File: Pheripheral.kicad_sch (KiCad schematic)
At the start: 19 parts

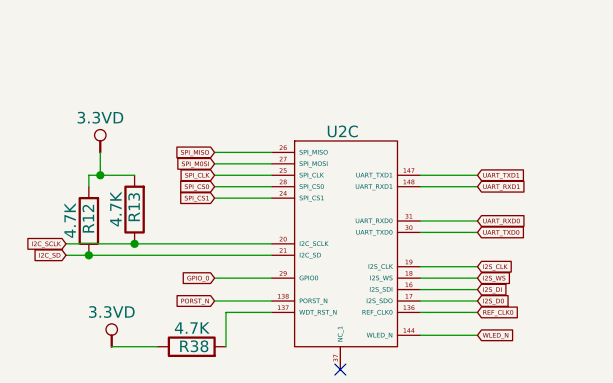
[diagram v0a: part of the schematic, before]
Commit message: f_ver
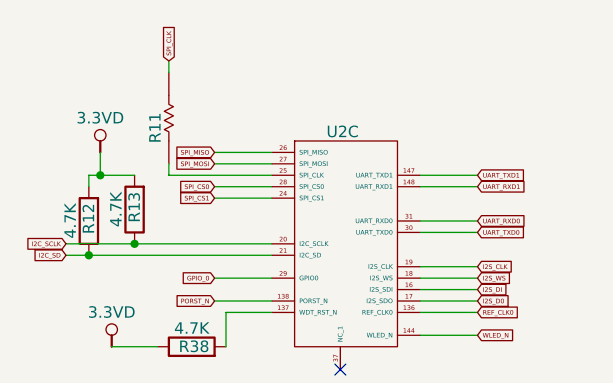
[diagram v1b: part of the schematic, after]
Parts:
- added R11: 22, Resistor_SMD:R_0402_1005Metric, symbol MT7688AN_Reset-altium-import:root_2_Res1_Miscellaneous Devices.SchLib
- U2: footprint MT7628:MT7628_footprint -> Library:MT7628_footprint
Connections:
- net SPI_CLK: now also R11.1; no longer U2.25 (SPI_CLK)
- net SPI_M0SI renamed SPI_MOSI
- new net: R11.2, U2.25 (SPI_CLK)
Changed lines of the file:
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@@
 	(wire
 		(pts
+			(xy 43.18 29.21) (xy 43.18 30.48)
+		)
+		(stroke
+			(width 0)
+			(type default)
+		)
+	)
+	(wire
+		(pts
 			(xy 31.75 39.37) (xy 34.29 39.37)
 		)
@@
 	(wire
 		(pts
+			(xy 43.18 17.78) (xy 43.18 19.05)
+		)
+		(stroke
+			(width 0)
+			(type default)
+		)
+	)
+	(wire
+		(pts
 			(xy 115.57 34.29) (xy 127 34.29)
 		)
@@
 	(wire
 		(pts
+			(xy 43.18 30.48) (xy 54.61 30.48)
+		)
+		(stroke
+			(width 0)
+			(type default)
+		)
+	)
+	(wire
+		(pts
 			(xy 149.86 29.21) (xy 152.4 29.21)
 		)
@@
 	(wire
 		(pts
-			(xy 48.26 30.48) (xy 54.61 30.48)
-		)
-		(stroke
-			(width 0)
-			(type default)
-		)
-	)
-	(wire
-		(pts
 			(xy 48.26 33.02) (xy 54.61 33.02)
 		)
@@
 		)
 	)
-	(global_label "SPI_M0SI"
+	(global_label "SPI_MOSI"
 		(shape input)
 		(at 48.26 29.21 180)
@@
 		)
 		(property "Intersheetrefs" "${INTERSHEET_REFS}"
-			(at 43.6551 29.21 0)
+			(at 43.6067 29.21 0)
 			(effects
 				(font
@@
 	(global_label "SPI_CLK"
 		(shape input)
-		(at 48.26 30.48 180)
+		(at 43.18 17.78 90)
 		(fields_autoplaced yes)
 		(effects
@@
 				(size 0.508 0.508)
 			)
-			(justify right)
+			(justify left)
 		)
 		(property "Intersheetrefs" "${INTERSHEET_REFS}"
-			(at 44.018 30.48 0)
+			(at 43.18 13.538 90)
 			(effects
 				(font
 					(size 1.27 1.27)
 				)
-				(justify right)
+				(justify left)
 				(hide yes)
 			)
@@
 			)
 		)
-		(property "Footprint" "MT7628:MT7628_footprint"
+		(property "Footprint" "Library:MT7628_footprint"
 			(at 62.23 27.94 0)
 			(effects
@@
 			)
 		)
-		(property "Footprint" "MT7628:MT7628_footprint"
+		(property "Footprint" "Library:MT7628_footprint"
 			(at 163.83 43.18 0)
 			(effects
@@
 	)
 	(symbol
+		(lib_id "MT7688AN_Reset-altium-import:root_2_Res1_Miscellaneous Devices.SchLib")
+		(at 45.72 21.59 90)
+		(unit 1)
+		(exclude_from_sim no)
+		(in_bom yes)
+		(on_board yes)
+		(dnp no)
+		(property "Reference" "R11"
+			(at 42.418 26.924 0)
+			(effects
+				(font
+					(size 1.27 1.27)
+				)
+				(justify left bottom)
+			)
+		)
+		(property "Value" "22"
+			(at 42.418 29.718 0)
+			(effects
+				(font
+					(size 1.27 1.27)
+				)
+				(justify left bottom)
+				(hide yes)
+			)
+		)
+		(property "Footprint" "Resistor_SMD:R_0402_1005Metric"
+			(at 45.72 21.59 0)
+			(effects
+				(font
+					(size 1.27 1.27)
+				)
+				(hide yes)
+			)
+		)
+		(property "Datasheet" ""
+			(at 45.72 21.59 0)
+			(effects
+				(font
+					(size 1.27 1.27)
+				)
+				(hide yes)
+			)
+		)
+		(property "Description" "Resistor"
+			(at 45.72 21.59 0)
+			(effects
+				(font
+					(size 1.27 1.27)
+				)
+				(hide yes)
+			)
+		)
+		(property "PUBLISHED" "8-Jun-2000"
+			(at 42.418 29.718 0)
+			(effects
+				(font
+					(size 1.27 1.27)
+				)
+				(justify left bottom)
+				(hide yes)
+			)
+		)
+		(property "LATESTREVISIONDATE" "17-Jul-2002"
+			(at 42.418 29.718 0)
+			(effects
+				(font
+					(size 1.27 1.27)
+				)
+				(justify left bottom)
+				(hide yes)
+			)
+		)
+		(property "LATESTREVISIONNOTE" "Re-released for DXP Platform."
+			(at 42.418 29.718 0)
+			(effects
+				(font
+					(size 1.27 1.27)
+				)
+				(justify left bottom)
+				(hide yes)
+			)
+		)
+		(property "PACKAGEREFERENCE" "AXIAL-0.3"
+			(at 42.418 29.718 0)
+			(effects
+				(font
+					(size 1.27 1.27)
+				)
+				(justify left bottom)
+				(hide yes)
+			)
+		)
+		(property "PUBLISHER" "Altium Limited"
+			(at 42.418 29.718 0)
+			(effects
+				(font
+					(size 1.27 1.27)
+				)
+				(justify left bottom)
+				(hide yes)
+			)
+		)
+		(property "PACKAGEDESCRIPTION" "Axial Device, Thru-Hole; 2 Leads; 0.3 in Pin Spacing"
+			(at 42.418 29.718 0)
+			(effects
+				(font
+					(size 1.27 1.27)
+				)
+				(justify left bottom)
+				(hide yes)
+			)
+		)
+		(property "ALTIUM_VALUE" "22¦¸"
+			(at 46.482 26.924 0)
+			(effects
+				(font
+					(size 1.27 1.27)
+				)
+				(justify left bottom)
+				(hide yes)
+			)
+		)
+		(property "LCSC" "C25092"
+			(at 45.72 21.59 0)
+			(effects
+				(font
+					(size 1.27 1.27)
+				)
+				(hide yes)
+			)
+		)
+		(pin "2"
+		)
+		(pin "1"
+		)
+		(instances
+			(project "mt7628v1"
+				(path "/144686d4-2b77-460c-9924-cc86faff7e9d/218ba002-e319-46e9-a80e-651bdbb44c2c"
+					(reference "R11")
+					(unit 1)
+				)
+			)
+		)
+	)
+	(symbol
 		(lib_id "Device:C")
 		(at 88.9 93.98 0)
@@
 			)
 		)
-		(property "Footprint" "MT7628:MT7628_footprint"
+		(property "Footprint" "Library:MT7628_footprint"
 			(at 124.46 99.06 0)
 			(effects
